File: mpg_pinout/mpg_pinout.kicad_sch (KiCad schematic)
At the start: 9 parts, among them J1 Conn_02x05_Odd_Even, J2 Conn_01x02_Pin, J3 Conn_01x02_Pin, J4 Conn_01x02_Pin, J5 Conn_01x02_Pin, J6 Conn_01x02_Pin, J7 Conn_01x02_Pin, J8 Conn_01x02_Pin

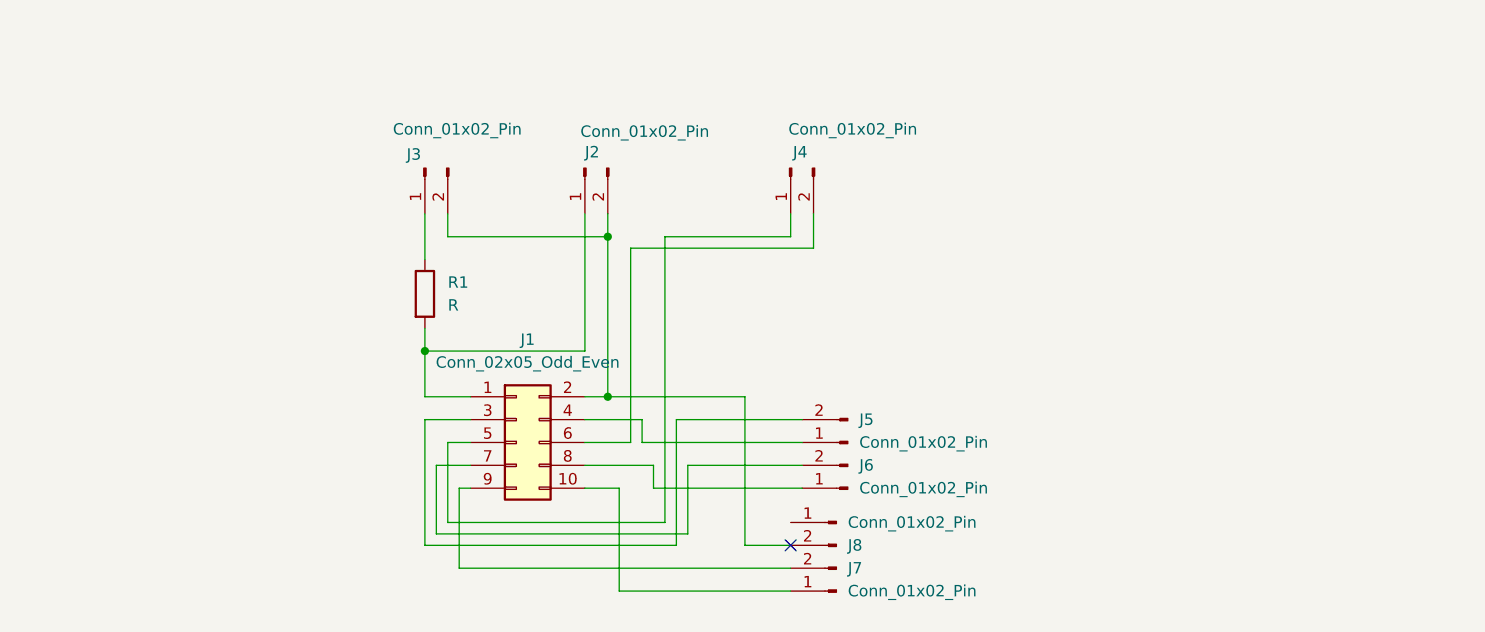
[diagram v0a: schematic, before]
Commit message: third commit
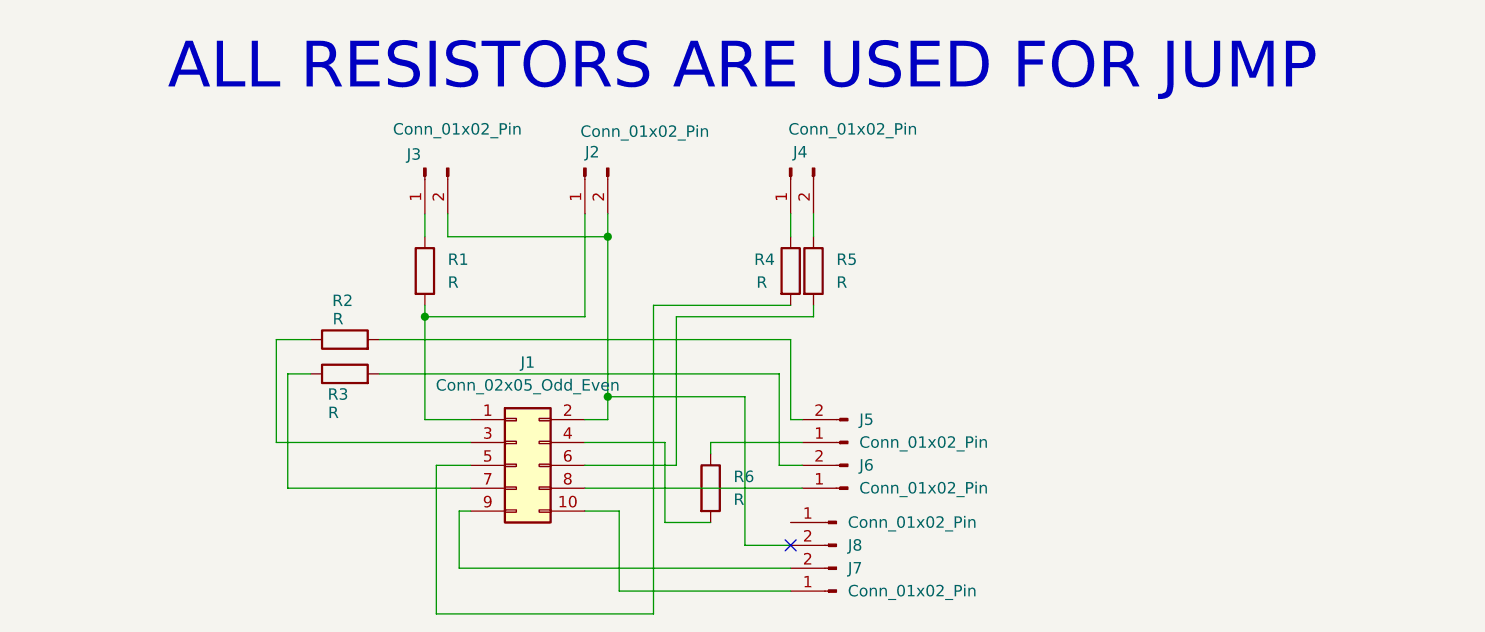
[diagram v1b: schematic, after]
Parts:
- added R2, R3, R5, R6: R, Resistor_THT:R_Axial_DIN0414_L11.9mm_D4.5mm_P15.24mm_Horizontal, symbol Device:R
- added R4: R, Resistor_THT:R_Axial_DIN0414_L11.9mm_D4.5mm_P25.40mm_Horizontal, symbol Device:R
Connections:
- net at J5.1 (Pin_1): now also R6.1; no longer J1.4 (Pin_4)
- net at J5.2 (Pin_2): now also R2.2; no longer J1.3 (Pin_3)
- net at J4.1 (Pin_1): now also R4.1; no longer J1.5 (Pin_5)
- net at J4.2 (Pin_2): now also R5.1; no longer J1.6 (Pin_6)
- net at J1.7 (Pin_7): now also R3.1; no longer J6.2 (Pin_2)
- new net: J6.2 (Pin_2), R3.2
- new net: J1.3 (Pin_3), R2.1
- new net: J1.4 (Pin_4), R6.2
- new net: J1.5 (Pin_5), R4.2
- new net: J1.6 (Pin_6), R5.2
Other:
- note added: "ALL RESISTORS ARE USED FOR JUMP"
- moved on the sheet: J1, R1
